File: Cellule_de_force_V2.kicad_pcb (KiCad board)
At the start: 2 copper layers, 26.9 x 68.1 mm, 70 parts, among them IC2 TPS61086DRCR, J1 Conn_01x02_Pin, J2 Conn_01x02_Pin, J3 Conn_01x02_Pin, J4 Conn_01x02_Pin, J5 Conn_01x04_Socket, J6 Conn_01x05_Pin, U1 AD7190WBRUZ, U2 LT3042IMSE, Y1 ABC2-4.9152MHZ-4-T

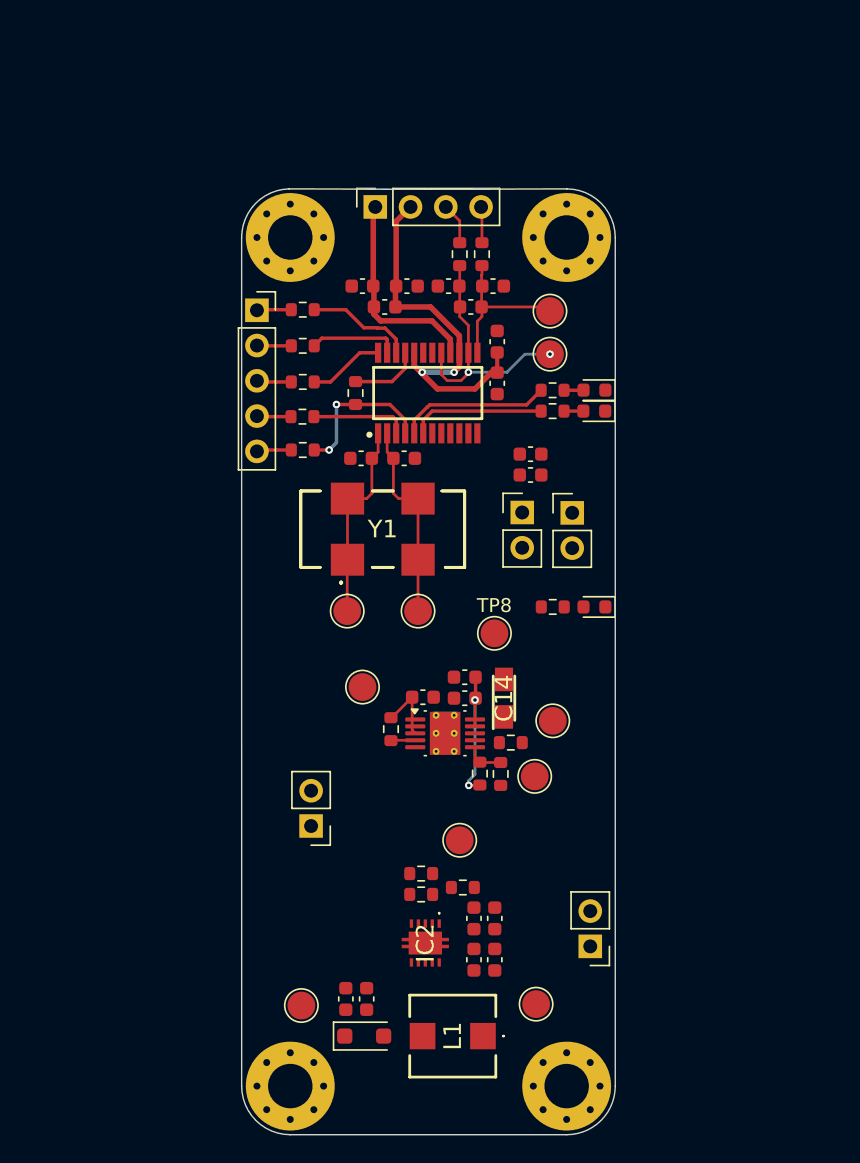
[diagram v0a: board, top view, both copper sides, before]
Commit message: [PCB 4 layer]
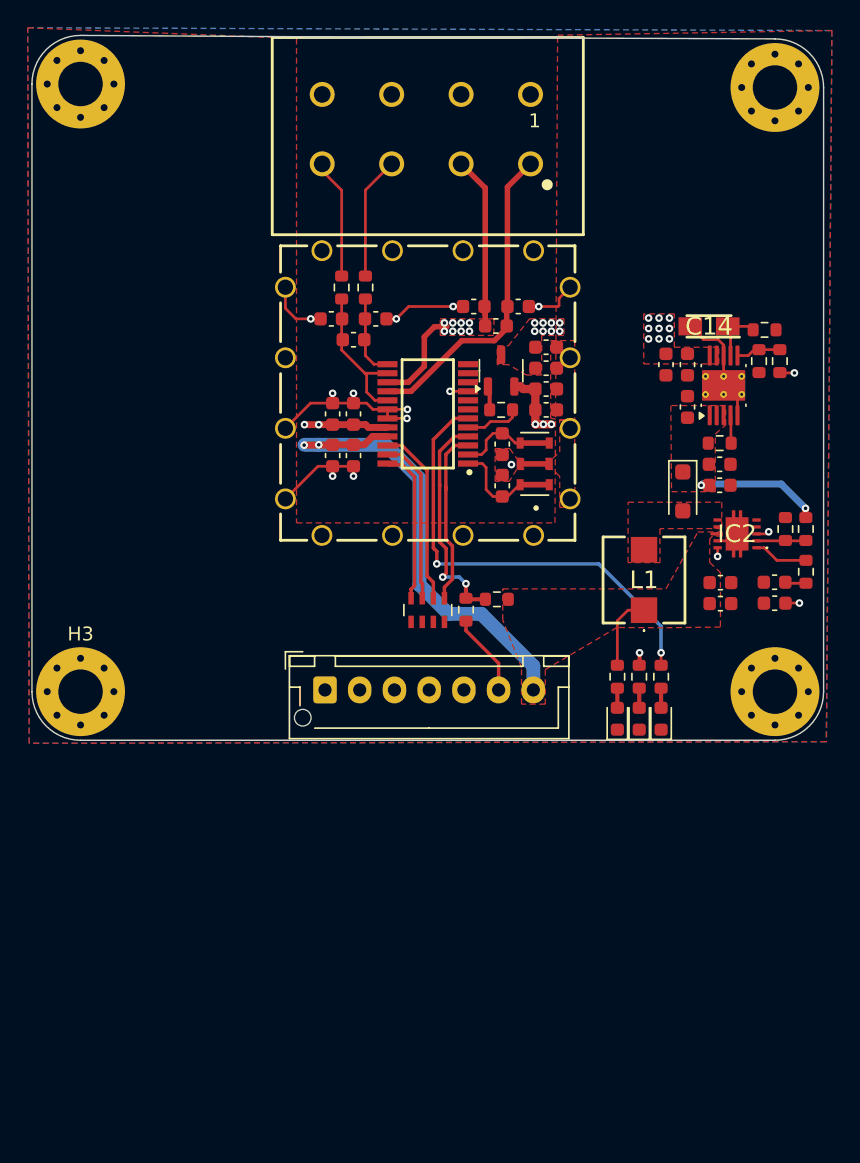
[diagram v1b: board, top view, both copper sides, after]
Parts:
- removed J2, J4: Conn_01x02_Pin, Connector_PinHeader_2.54mm:PinHeader_1x02_P2.54mm_Vertical
- removed J5: Conn_01x04_Socket, Connector_PinSocket_2.54mm:PinSocket_1x04_P2.54mm_Vertical
- removed J6: Conn_01x05_Pin, Connector_PinSocket_2.54mm:PinSocket_1x05_P2.54mm_Vertical
- removed R4, R5, R7: 100Ω, Resistor_SMD:R_0603_1608Metric
- removed TP14, TP15, TP16, TP17, TP18, TP19, TP20, TP3, TP4, TP6, TP8: TestPoint, TestPoint:TestPoint_Pad_D2.0mm
- removed Y1: ABC2-4.9152MHZ-4-T, ABC2-4.9152MHZ-4-T:ABC210000MHZ4
- added C23: 0.1µF, Capacitor_SMD:C_0603_1608Metric, F.Cu at (157.0, 86.7)
- added C24: 18pf, Capacitor_SMD:C_0603_1608Metric, F.Cu at (153.9, 93.7)
- added C25: 18pf, Capacitor_SMD:C_0603_1608Metric, F.Cu at (153.9, 96.7)
- added C26: 0.1µF, Capacitor_SMD:C_0603_1608Metric, F.Cu at (157.0, 91.2)
- added H5: WE-SHC_THT-FRAME, WE-SHC_THT-FRAME:WE-SHC_THT-FRAME_36503205, F.Cu at (148.5, 90.0)
- added Q1: SI2303CDS-T1-GE3, Package_TO_SOT_SMD:SOT-23-3, F.Cu at (153.8, 88.4)
- added RN1: RP_100Ω, Resistor_SMD:R_Array_Concave_4x0603, F.Cu at (148.5, 105.6)
- added Y2: CSTCR4M91G53-R0, CSTCR4M91G53-R0:OSC_CSTCR4M91G53-R0, F.Cu at (156.2, 95.1)
- C11: value 22pf -> 0.1µF
- C12: value 22pf -> 10µF
- D2: value LED -> RED
- J1: value Conn_01x02_Pin -> Conn_01x07_Pin; footprint Connector_PinHeader_2.54mm:PinHeader_1x02_P2.54mm_Vertical -> Connector_JST:JST_XH_B7B-XH-AM_1x07_P2.50mm_Vertical
- J3: value Conn_01x02_Pin -> 691408720004B; footprint Connector_PinHeader_2.54mm:PinHeader_1x02_P2.54mm_Vertical -> 691408720004B:691408720004B
- R10: value 100Ω -> 1kΩ
- moved C20 47.0 mm to (169.5, 95.1), turned to 0 degrees
- moved D3 45.4 mm to (166.9, 97.1), turned to -90 degrees
- moved C19 44.9 mm to (169.5, 96.6), turned to 0 degrees
- moved R17 37.2 mm to (175.7, 99.8), turned to 90 degrees
- moved R15 37.1 mm to (174.2, 99.8), turned to -90 degrees
- moved IC2 37.0 mm to (170.8, 100.1), turned to 180 degrees
- moved R12 36.7 mm to (173.8, 87.7)
- moved L1 35.6 mm to (164.1, 103.5), turned to 180 degrees
- moved R13 35.1 mm to (172.3, 87.7)
- moved R9 34.9 mm to (172.8, 85.5)
- moved R18 33.6 mm to (175.7, 102.9), turned to 90 degrees
- moved C17 32.5 mm to (173.5, 103.6), turned to 180 degrees
- moved C22 32.4 mm to (169.6, 103.7), turned to 0 degrees
- moved H3 32.2 mm to (123.5, 111.5)
- moved H4 32.1 mm to (173.5, 111.5)
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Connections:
- net Net-(U1-P3) renamed P3
- C1 pad 1: +3.3V_IN -> +3.3V
- C11 pad 1: MCLK2 -> SENSE+
- C12 pad 1: MCLK1 -> +5VA
- C13 pad 1: +5VA_OUT -> +5VA
- C15 pad 1: +5VA_OUT -> +5VA
- C16 pad 1: +6V_IN -> +6V
- C19 pad 1: +6V_OUT -> +6V
- C2 pad 1: +3.3V_IN -> +3.3V
- C20 pad 1: +6V_OUT -> +6V
- C21 pad 1: +3.3V_IN -> +3.3V
- C22 pad 1: +3.3V_IN -> +3.3V
- C3 pad 2: IN-SENSE+ -> +5VA
- C4 pad 2: IN-SENSE+ -> +5VA
- C5 pad 1: IN-SENSE+ -> SENSE+
- C5 pad 2: IN-SENSE- -> SENSE-
- C7 pad 2: IN-SENSE+ -> SENSE+
- C9 pad 1: IN-SENSE- -> SENSE-
- D3 pad 1: +6V_OUT -> +6V
- IC2 pad 3: +3.3V_IN -> +3.3V
- IC2 pad 8: +3.3V_IN -> +3.3V
- J1 pad 1: +3.3V_IN -> GND
- J1 pad 2: GND -> DOUT
- J3 pad 1: +3.3V_IN -> SENSE-
- J3 pad 2: +3.3V_IN -> SENSE+
- L1 pad 1: +3.3V_IN -> +3.3V
- R10 pad 2: Net-(D1-A) -> Net-(Q1-G)
- R12 pad 2: +5VA_OUT -> +5VA
- R14 pad 1: +6V_IN -> +6V
- R16 pad 2: +5VA_OUT -> +5VA
- R17 pad 2: +6V_OUT -> +6V
- R3 pad 1: DIN -> Net-(D1-A)
- R3 pad 2: Net-(U1-DIN) -> +3.3V
- R8 pad 1: +3.3V_IN -> +3.3V
- U1 pad 15: IN-SENSE+ -> SENSE+
- U1 pad 16: IN-SENSE- -> SENSE-
- U1 pad 20: IN-SENSE+ -> +5VA
- U1 pad 21: +3.3V_IN -> +3.3V
- U1 pad 24: Net-(U1-DIN) -> Net-(RN1-R4.1)
- U1 pad 9: (no net) -> GND
- U2 pad 1: +6V_IN -> +6V
- U2 pad 10: +5VA_OUT -> +5VA
- U2 pad 2: +6V_IN -> +6V
- U2 pad 3: +6V_IN -> +6V
- U2 pad 9: +5VA_OUT -> +5VA
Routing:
- net GND: track 0.02 -> 46.4 mm, vias 0 -> 12
- net +3.3V: track 0.00 -> 42.4 mm, vias 0 -> 3
- net IN-SENSE+: track 27.8 -> 0.00 mm, vias 2 -> 0
- net Net-(U1-P2): track 9.71 -> 33.1 mm, vias 0 -> 2
- net SENSE-: track 0.00 -> 23.0 mm
- net SENSE+: track 0.00 -> 20.1 mm, vias 0 -> 16
- net IN-SENSE-: track 15.0 -> 0.00 mm
- net +5VA: track 0.00 -> 13.3 mm, vias 0 -> 16
- net Net-(RN1-R4.1): track 0.00 -> 11.1 mm
- net +5VA_OUT: track 10.6 -> 0.00 mm, vias 2 -> 0
- net +6V: track 0.00 -> 9.50 mm, vias 0 -> 2
- net MCLK2: track 14.5 -> 6.13 mm
- net OUT-: track 18.4 -> 10.8 mm, vias 2 -> 0
- net MCLK1: track 14.6 -> 7.07 mm
- net P3: track 11.0 -> 4.04 mm
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- added copper zone on F.Cu, net +3.3V
- added copper zone on F.Cu, net +5VA
- added copper zone on In2.Cu, net +5VA
- added copper zone on F.Cu, net +6V
- added copper zone on B.Cu, net GND
- added copper zone on F.Cu, net GND
- added copper zone on In1.Cu, net GND
- added copper zone on F.Cu, net Net-(D3-A)
- added copper zone on F.Cu, net SENSE+
- added copper zone on In2.Cu, net SENSE+
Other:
- board size 26.9 x 68.1 mm -> 57 x 50.8 mm
- copper layers 2 -> 4
